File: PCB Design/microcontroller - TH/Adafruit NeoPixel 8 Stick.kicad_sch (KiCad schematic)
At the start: 7 parts, among them CN2 1X4SMT, U1 ATmega328P-P, Y1 Crystal_Small

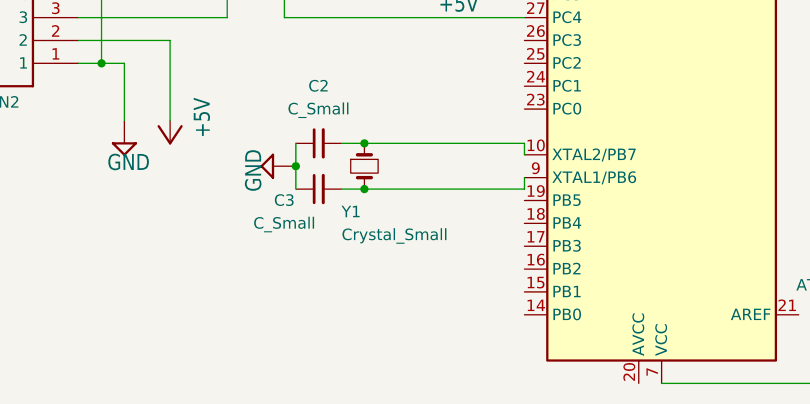
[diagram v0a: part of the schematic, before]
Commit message: updated some pcbs
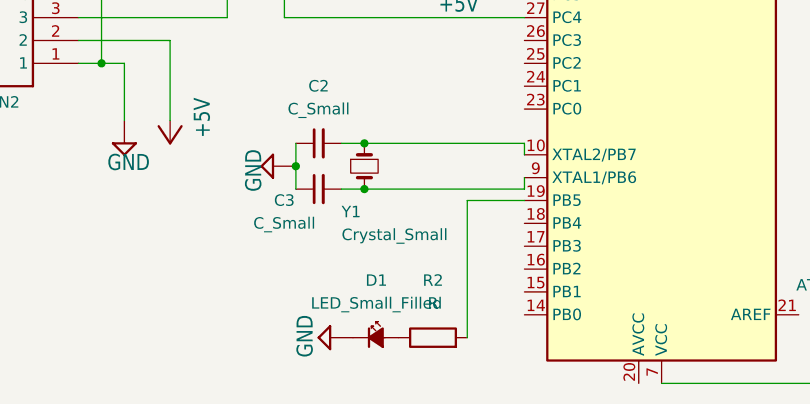
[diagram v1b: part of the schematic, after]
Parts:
- added D1: LED_Small_Filled, LED_THT:LED_D3.0mm, symbol Device:LED_Small_Filled
- added R2: R, Resistor_THT:R_Axial_DIN0207_L6.3mm_D2.5mm_P7.62mm_Horizontal, symbol Device:R
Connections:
- net GND: now also D1.1 (K)
- net at U1.19 (PB5): now also R2.2
- new net: D1.2 (A), R2.1
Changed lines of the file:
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@@
+    (stroke (width 0) (type default) (color 0 0 0 0))
+  )
+  (wire (pts (xy 90.17 142.24) (xy 83.82 142.24))
     (stroke (width 0) (type default) (color 0 0 0 0))
   )
@@
   )
   (wire (pts (xy 64.77 135.89) (xy 64.77 138.43))
+    (stroke (width 0) (type default) (color 0 0 0 0))
+  )
+  (wire (pts (xy 83.82 142.24) (xy 83.82 157.48))
     (stroke (width 0) (type default) (color 0 0 0 0))
   )
@@
     (pin "2")
   )
+  (symbol (lib_id "Adafruit NeoPixel 8 Stick-eagle-import:GND") (at 68.58 157.48 270) (unit 1)
+    (in_bom yes) (on_board yes)
+    (property "Reference" "#SUPPLY0103" (id 0) (at 68.58 157.48 0)
+      (effects (font (size 1.27 1.27)) hide)
+    )
+    (property "Value" "GND" (id 1) (at 64.77 154.94 0)
+      (effects (font (size 1.778 1.5113)) (justify left bottom))
+    )
+    (property "Footprint" "Adafruit NeoPixel 8 Stick:" (id 2) (at 68.58 157.48 0)
+      (effects (font (size 1.27 1.27)) hide)
+    )
+    (property "Datasheet" "" (id 3) (at 68.58 157.48 0)
+      (effects (font (size 1.27 1.27)) hide)
+    )
+    (pin "1")
+  )
   (symbol (lib_id "Device:C_Small") (at 67.31 140.97 90) (unit 1)
     (in_bom yes) (on_board yes)
@@
     (pin "2")
   )
+  (symbol (lib_id "Device:R") (at 80.01 157.48 90) (unit 1)
+    (in_bom yes) (on_board yes) (fields_autoplaced)
+    (property "Reference" "R2" (id 0) (at 80.01 151.13 90))
+    (property "Value" "R" (id 1) (at 80.01 153.67 90))
+    (property "Footprint" "Resistor_THT:R_Axial_DIN0207_L6.3mm_D2.5mm_P7.62mm_Horizontal" (id 2) (at 80.01 159.258 90)
+      (effects (font (size 1.27 1.27)) hide)
+    )
+    (property "Datasheet" "~" (id 3) (at 80.01 157.48 0)
+      (effects (font (size 1.27 1.27)) hide)
+    )
+    (pin "1")
+    (pin "2")
+  )
   (symbol (lib_id "Device:Crystal_Small") (at 72.39 138.43 270) (unit 1)
     (in_bom yes) (on_board yes)
@@
     )
     (property "Datasheet" "~" (id 3) (at 72.39 138.43 0)
+      (effects (font (size 1.27 1.27)) hide)
+    )
+    (pin "1")
+    (pin "2")
+  )
+  (symbol (lib_id "Device:LED_Small_Filled") (at 73.66 157.48 0) (unit 1)
+    (in_bom yes) (on_board yes) (fields_autoplaced)
+    (property "Reference" "D1" (id 0) (at 73.7235 151.13 0))
+    (property "Value" "LED_Small_Filled" (id 1) (at 73.7235 153.67 0))
+    (property "Footprint" "LED_THT:LED_D3.0mm" (id 2) (at 73.66 157.48 90)
+      (effects (font (size 1.27 1.27)) hide)
+    )
+    (property "Datasheet" "~" (id 3) (at 73.66 157.48 90)
       (effects (font (size 1.27 1.27)) hide)
     )
@@
       (reference "#SUPPLY0102") (unit 1) (value "GND") (footprint "Adafruit NeoPixel 8 Stick:")
     )
+    (path "/d224a906-f58c-46d7-8992-04eb3de8c733"
+      (reference "#SUPPLY0103") (unit 1) (value "GND") (footprint "Adafruit NeoPixel 8 Stick:")
+    )
     (path "/4f244128-34c9-469c-9b8c-59cd56544a99"
       (reference "#SUPPLY0104") (unit 1) (value "GND") (footprint "Adafruit NeoPixel 8 Stick:")
@@
       (reference "CN2") (unit 1) (value "1X4SMT") (footprint "Adafruit NeoPixel 8 Stick:1X4-SMT")
     )
+    (path "/ff207611-48ef-462c-aae3-a0e75d2a76d8"
+      (reference "D1") (unit 1) (value "LED_Small_Filled") (footprint "LED_THT:LED_D3.0mm")
+    )
     (path "/ca5547bc-940c-4718-9b74-8cc68e327ebd"
       (reference "R1") (unit 1) (value "R") (footprint "Resistor_THT:R_Axial_DIN0207_L6.3mm_D2.5mm_P7.62mm_Horizontal")
     )
+    (path "/d99a1d06-5b89-4f3c-b111-4ef4580f1358"
+      (reference "R2") (unit 1) (value "R") (footprint "Resistor_THT:R_Axial_DIN0207_L6.3mm_D2.5mm_P7.62mm_Horizontal")
+    )
     (path "/0930caa3-7c54-4b6e-8676-958f70cf0cd2"

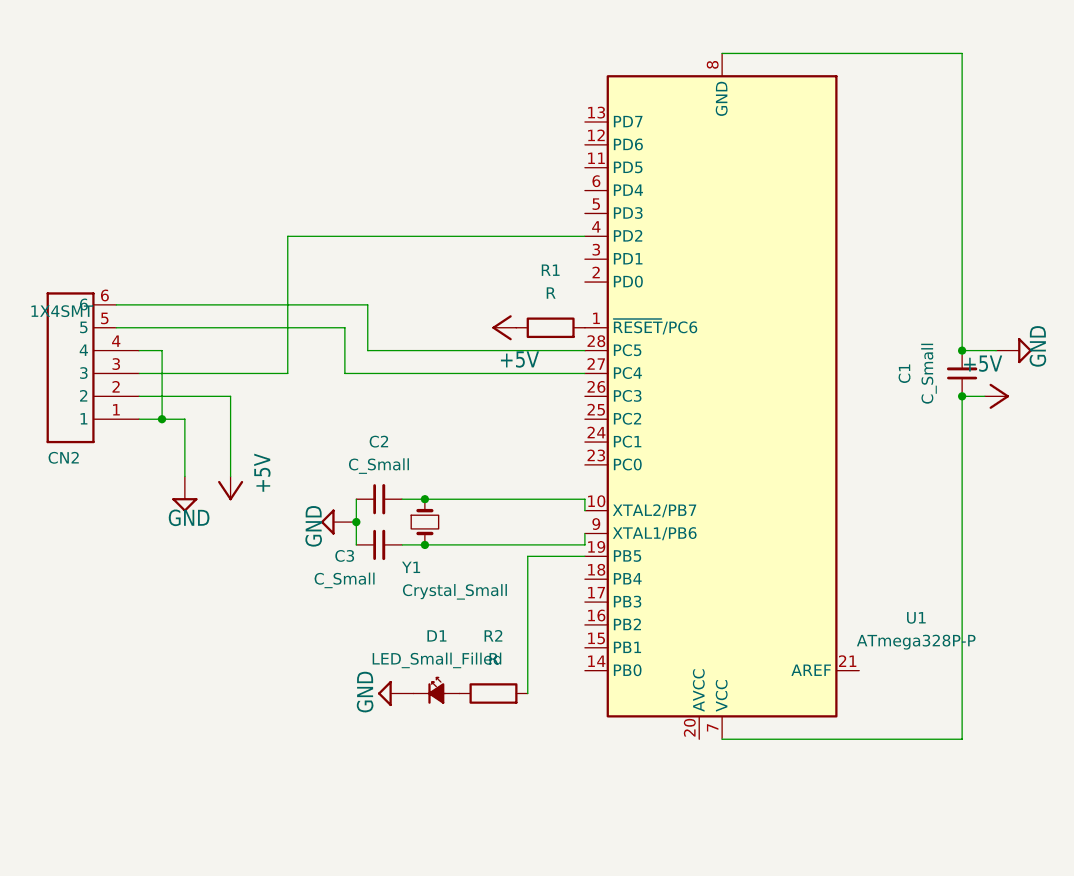
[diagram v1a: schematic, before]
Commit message: clean up boards + generate some gerber files
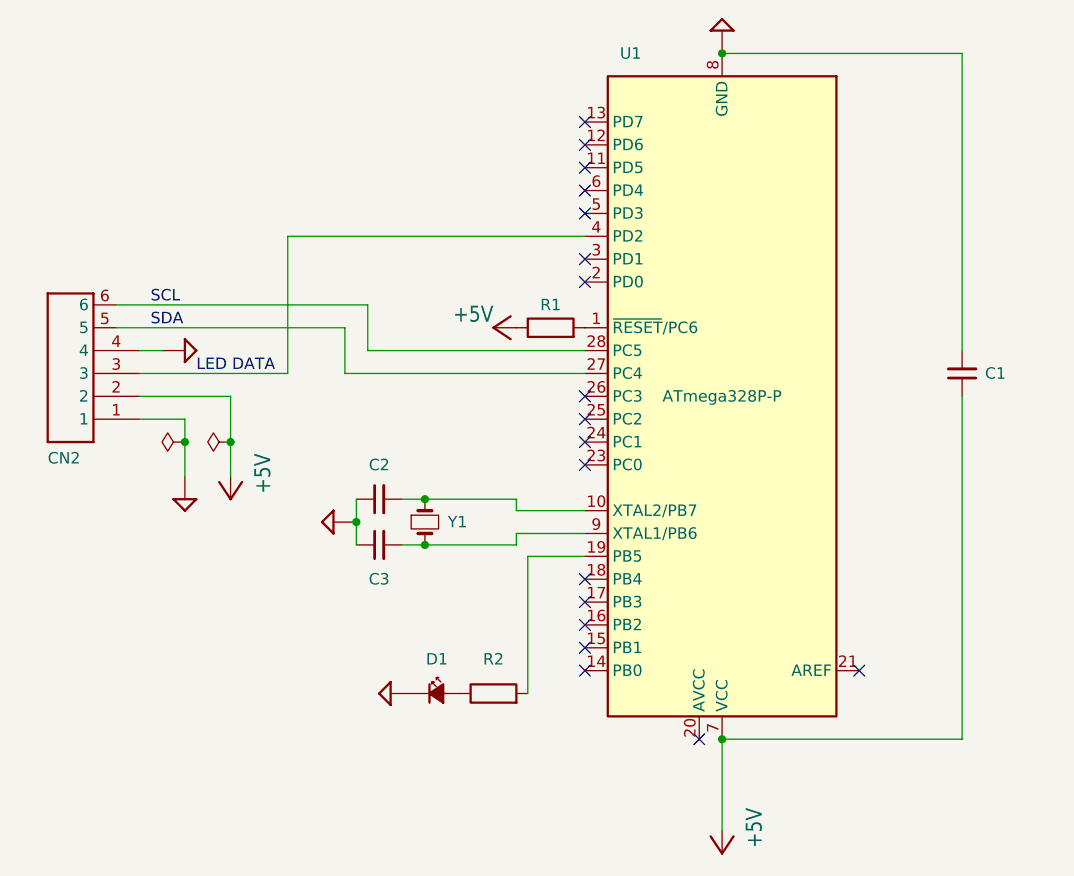
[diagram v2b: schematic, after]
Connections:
- net SDA: now reaches CN2.5, U1.27 (PC4)
- net SCL: now reaches CN2.6, U1.28 (PC5)
- net LED DATA: now reaches CN2.3, U1.4 (PD2)
- no-connect marks 0 -> 18
